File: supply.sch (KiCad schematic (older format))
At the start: 39 parts, among them J1 MJ-3536, J2 2, J3 3, J4 1, J5 GND, J6 Conn_01x01_Female, J7 Conn_01x01_Female, J8 Conn_01x01_Female, J9 Conn_01x01_Female, SW1 TE6-1A-DC-1-PB, U1 LM5157, U2 LM386

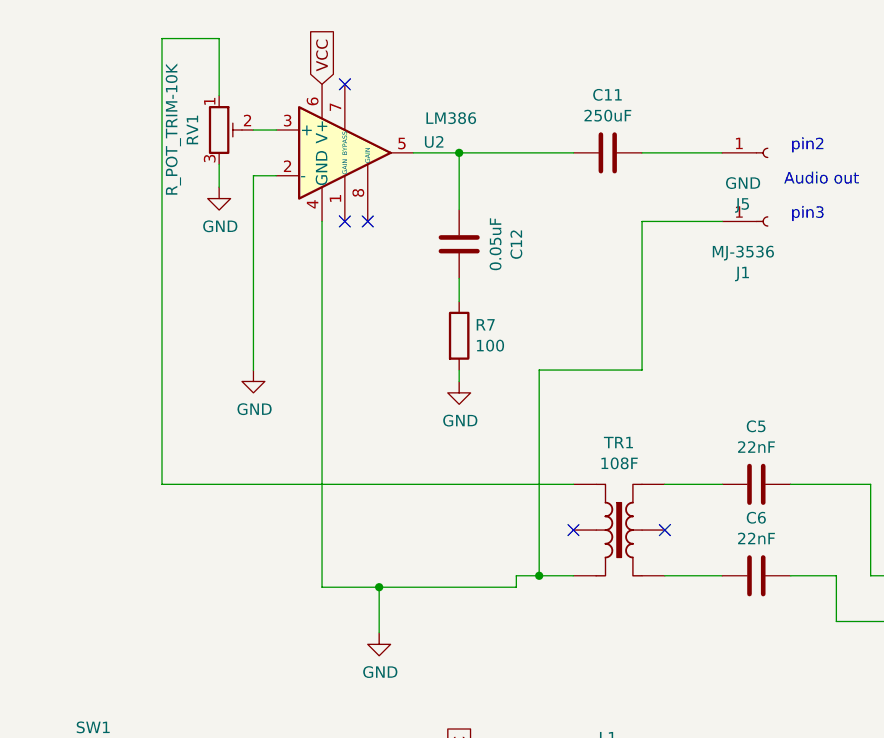
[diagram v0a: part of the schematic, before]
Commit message: Add files via upload
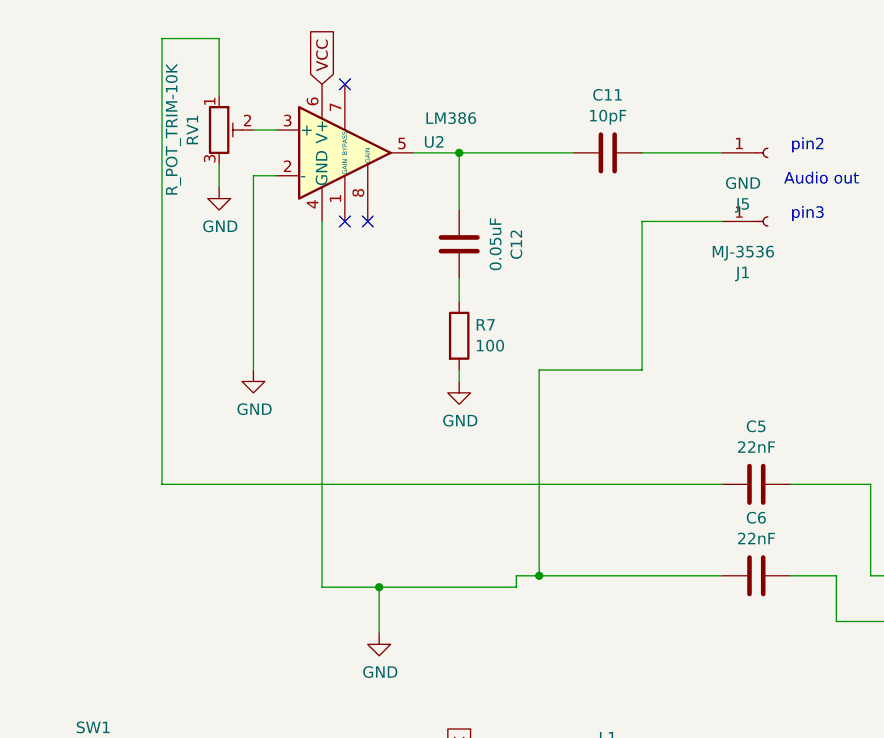
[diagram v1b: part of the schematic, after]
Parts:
- removed TR1: 108F, supply:108F, symbol Transformer:TRANSF5
- C11: value 250uF -> 10pF
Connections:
- net GND: now also C6.2
- net at C5.2: now also RV1.1
- no-connect marks 7 -> 5
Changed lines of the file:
@@
 Wire Wire Line
 	1250 4500 1250 5050
-$Comp
-L Transformer:TRANSF5 TR1
-U 1 1 60C979BB
-P 4600 2700
-F 0 "TR1" H 4600 3081 50  0000 C CNN
-F 1 "108F" H 4600 2990 50  0000 C CNN
-F 2 "supply:108F" H 4600 2700 50  0001 C CNN
-F 3 "" H 4600 2700 50  0001 C CNN
-	1    4600 2700
-	1    0    0    -1
-$EndComp
-Wire Wire Line
-	4800 2900 5050 2900
-NoConn ~ 4400 2700
-NoConn ~ 4800 2700
-Wire Wire Line
-	4800 2500 5050 2500
 Wire Wire Line
 	5350 2500 5700 2500
@@
 pin3
 Wire Wire Line
-	2600 2500 4400 2500
-Wire Wire Line
 	3550 2950 3300 2950
 Connection ~ 3550 2950
@@
 $EndComp
 Wire Wire Line
-	4250 2900 4400 2900
-Wire Wire Line
 	4150 2900 4250 2900
 Connection ~ 4250 2900
@@
 P 4550 1050
 F 0 "C11" V 4298 1050 50  0000 C CNN
-F 1 "250uF" V 4389 1050 50  0000 C CNN
+F 1 "10pF" V 4389 1050 50  0000 C CNN
 F 2 "Capacitor_THT:C_Disc_D3.8mm_W2.6mm_P2.50mm" H 4588 900 50  0001 C CNN
 F 3 "~" H 4550 1050 50  0001 C CNN
@@
 	1    0    0    -1
 $EndComp
+Wire Wire Line
+	2600 2500 5050 2500
+Wire Wire Line
+	4250 2900 5050 2900
 $EndSCHEMATC

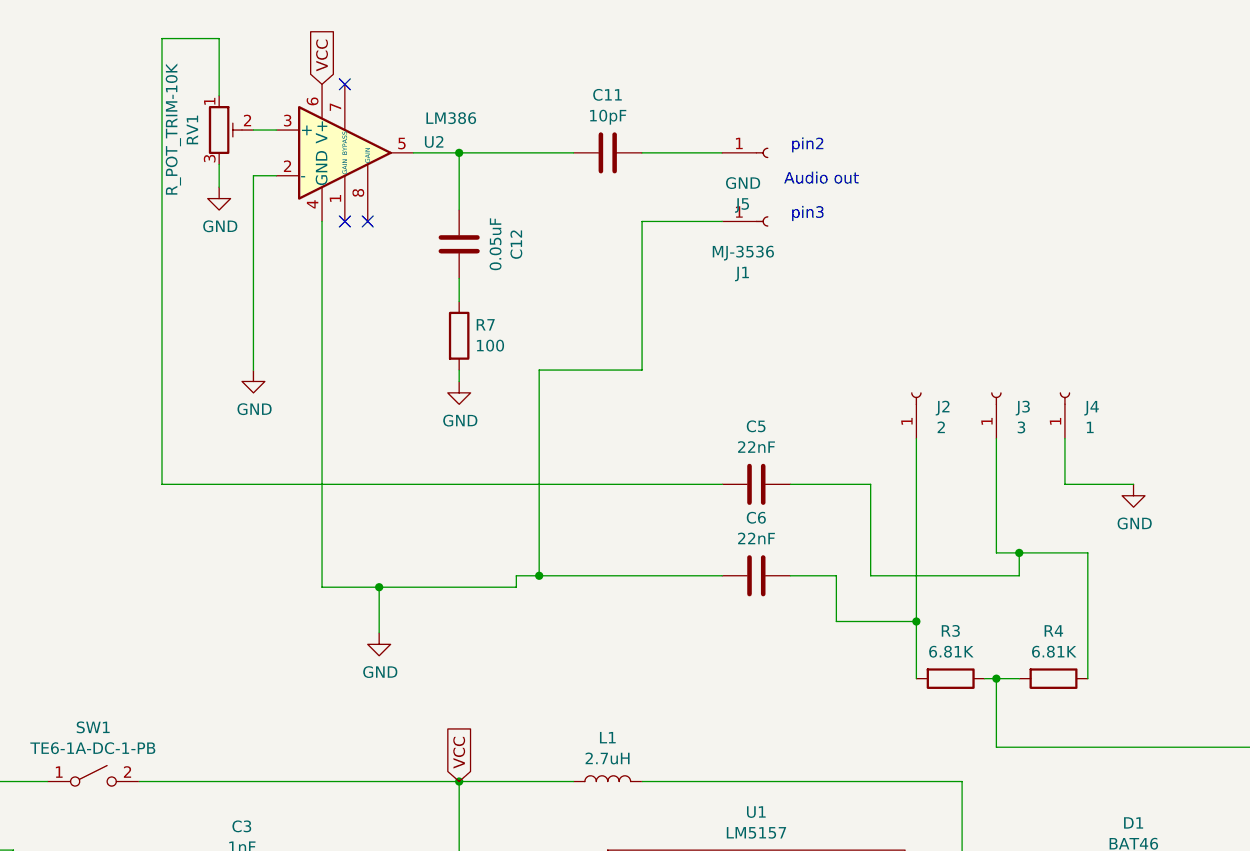
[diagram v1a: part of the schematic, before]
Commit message: Add files via upload
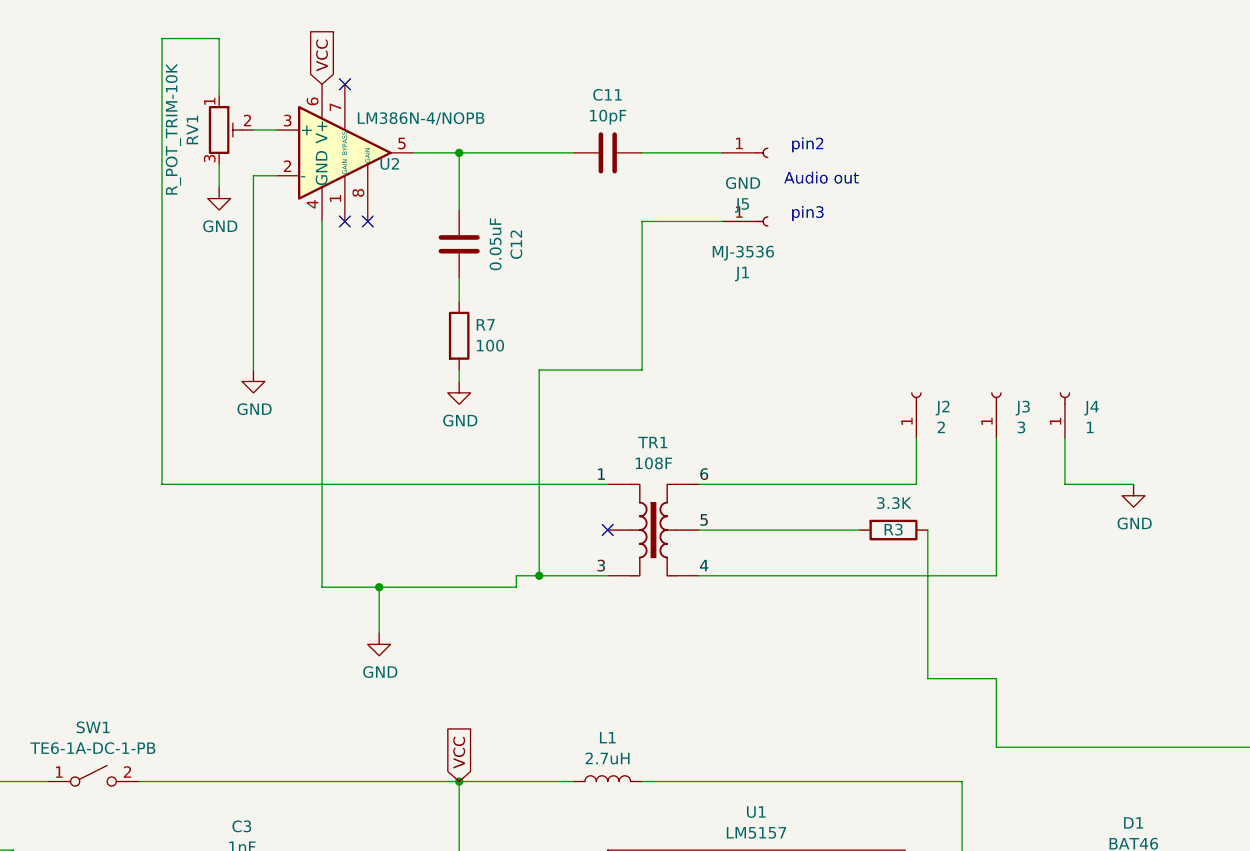
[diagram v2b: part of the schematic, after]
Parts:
- removed C5, C6: 22nF, Capacitor_THT:C_Disc_D3.8mm_W2.6mm_P2.50mm, symbol Device:C
- removed R4: 6.81K, Resistor_THT:R_Axial_DIN0207_L6.3mm_D2.5mm_P7.62mm_Horizontal, symbol Device:R
- added TR1: 108F, tastatur:108F, symbol Transformer:TRANSF5
- R3: value 6.81K -> 3.3K
- U2: value LM386 -> LM386N-4/NOPB
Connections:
- net GND: now also TR1.3
- net 5: now reaches R3.2
- net 5: now also TR1.5; no longer J2.1 (Pin_1)
- net 4: now reaches J3.1 (Pin_1)
- net 4: now also TR1.4
- net 1: now reaches RV1.1
- net 1: now also TR1.1
- new net 6: J2.1 (Pin_1), TR1.6
- no-connect marks 5 -> 6
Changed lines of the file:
@@
 Comment4 ""
 $EndDescr
-$Comp
-L Device:R R3
-U 1 1 60C4F601
-P 6050 3350
-F 0 "R3" V 5843 3350 50  0000 C CNN
-F 1 "6.81K" V 5934 3350 50  0000 C CNN
-F 2 "Resistor_THT:R_Axial_DIN0207_L6.3mm_D2.5mm_P7.62mm_Horizontal" V 5980 3350 50  0001 C CNN
-F 3 "~" H 6050 3350 50  0001 C CNN
-	1    6050 3350
-	0    1    1    0
-$EndComp
-$Comp
-L Device:R R4
-U 1 1 60C51D2E
-P 6500 3350
-F 0 "R4" V 6293 3350 50  0000 C CNN
-F 1 "6.81K" V 6384 3350 50  0000 C CNN
-F 2 "Resistor_THT:R_Axial_DIN0207_L6.3mm_D2.5mm_P7.62mm_Horizontal" V 6430 3350 50  0001 C CNN
-F 3 "~" H 6500 3350 50  0001 C CNN
-	1    6500 3350
-	0    1    1    0
-$EndComp
-Wire Wire Line
-	6650 3350 6650 2800
-Wire Wire Line
-	6650 2800 6350 2800
-Wire Wire Line
-	5900 3350 5900 3100
 Wire Wire Line
 	3550 2950 4150 2950
 Wire Wire Line
 	4150 2950 4150 2900
-Wire Wire Line
-	5550 2900 5550 3100
-Wire Wire Line
-	5550 3100 5900 3100
-Connection ~ 5900 3100
-$Comp
-L Device:C C6
-U 1 1 60C77EFA
-P 5200 2900
-F 0 "C6" V 4948 2900 50  0000 C CNN
-F 1 "22nF" V 5039 2900 50  0000 C CNN
-F 2 "Capacitor_THT:C_Disc_D3.8mm_W2.6mm_P2.50mm" H 5238 2750 50  0001 C CNN
-F 3 "~" H 5200 2900 50  0001 C CNN
-	1    5200 2900
-	0    1    1    0
-$EndComp
-Wire Wire Line
-	5550 2900 5350 2900
-Wire Wire Line
-	5700 2500 5700 2900
-Wire Wire Line
-	5700 2900 6350 2900
-Wire Wire Line
-	6350 2900 6350 2800
-Connection ~ 6350 2800
-Wire Wire Line
-	6350 2800 6250 2800
 $Comp
 L power:GND #PWR02
@@
 Wire Wire Line
 	1250 4500 1250 5050
-Wire Wire Line
-	5350 2500 5700 2500
-$Comp
-L Device:C C5
-U 1 1 60C76CC6
-P 5200 2500
-F 0 "C5" V 4948 2500 50  0000 C CNN
-F 1 "22nF" V 5039 2500 50  0000 C CNN
-F 2 "Capacitor_THT:C_Disc_D3.8mm_W2.6mm_P2.50mm" H 5238 2350 50  0001 C CNN
-F 3 "~" H 5200 2500 50  0001 C CNN
-	1    5200 2500
-	0    1    1    0
-$EndComp
 Text Notes 7150 6750 0    50   ~ 0
 Balanced power supply with mono headphone output jack.
@@
 $EndComp
 Wire Wire Line
-	6250 2300 6250 2800
-Wire Wire Line
 	6550 2500 6550 2300
 Text Notes 5650 1200 2    50   ~ 0
 Audio out
-Wire Wire Line
-	5900 2300 5900 3100
 $Comp
 L Connector:Conn_01x01_Female J6
@@
 	1    0    0    -1
 $EndComp
-Wire Wire Line
-	6200 3350 6250 3350
 $Comp
 L supply-rescue:LM5157-Keyboard U1
@@
 	6250 3650 6250 3350
 Connection ~ 8500 4200
-Connection ~ 6250 3350
-Wire Wire Line
-	6250 3350 6350 3350
 $Comp
 L Switch:SW_SPST SW1
@@
 U 1 1 60D34ED9
 P 3400 1050
-F 0 "U2" H 3744 1096 50  0000 L CNN
-F 1 "LM386" H 3750 1200 50  0000 L CNN
+F 0 "U2" H 3550 1000 50  0000 L CNN
+F 1 "LM386N-4/NOPB" H 3450 1200 50  0000 L CNN
 F 2 "Package_DIP:DIP-8_W7.62mm" H 3500 1150 50  0001 C CNN
 F 3 "http://www.ti.com/lit/ds/symlink/lm386.pdf" H 3600 1250 50  0001 C CNN
@@
 $EndComp
 Wire Wire Line
-	2600 2500 5050 2500
-Wire Wire Line
-	4250 2900 5050 2900
+	2600 2500 4550 2500
+Wire Wire Line
+	4250 2900 4550 2900
+$Comp
+L Device:R R3
+U 1 1 60D3C3AC
+P 5800 2700
+F 0 "R3" V 5800 2700 50  0000 C CNN
+F 1 "3.3K" V 5684 2700 50  0000 C CNN
+F 2 "Resistor_THT:R_Axial_DIN0207_L6.3mm_D2.5mm_P7.62mm_Horizontal" V 5730 2700 50  0001 C CNN
+F 3 "~" H 5800 2700 50  0001 C CNN
+	1    5800 2700
+	0    1    1    0
+$EndComp
+Wire Wire Line
+	5950 3350 5950 2700
+Wire Wire Line
+	5950 3350 6250 3350
+Wire Wire Line
+	6250 2300 6250 2900
+Wire Wire Line
+	5900 2500 5900 2300
+$Comp
+L Transformer:TRANSF5 TR1
+U 1 1 60D6EE08
+P 4750 2700
+F 0 "TR1" H 4750 3081 50  0000 C CNN
+F 1 "108F" H 4750 2990 50  0000 C CNN
+F 2 "tastatur:108F" H 4750 2700 50  0001 C CNN
+F 3 "" H 4750 2700 50  0001 C CNN
+	1    4750 2700
+	1    0    0    -1
+$EndComp
+Wire Wire Line
+	4950 2500 5900 2500
+Wire Wire Line
+	4950 2900 6250 2900
+Wire Wire Line
+	4950 2700 5650 2700
+NoConn ~ 4550 2700
+Text Label 4500 2500 0    50   ~ 0
+1
+Text Label 4500 2900 0    50   ~ 0
+3
+Text Label 4950 2500 0    50   ~ 0
+6
+Text Label 4950 2900 0    50   ~ 0
+4
+Text Label 4950 2700 0    50   ~ 0
+5
 $EndSCHEMATC
